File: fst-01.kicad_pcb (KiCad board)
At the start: 2 copper layers, 26.5 x 13.1 mm, 25 parts, among them J1 USB_A, K1 CONN_3, K2 CONN_2, K3 CONN_2, U1 STM32F103TB, U2 LP2985-33DBVR, U3 NUF2221W1, U4 SST25VF032B, X1 12MHz

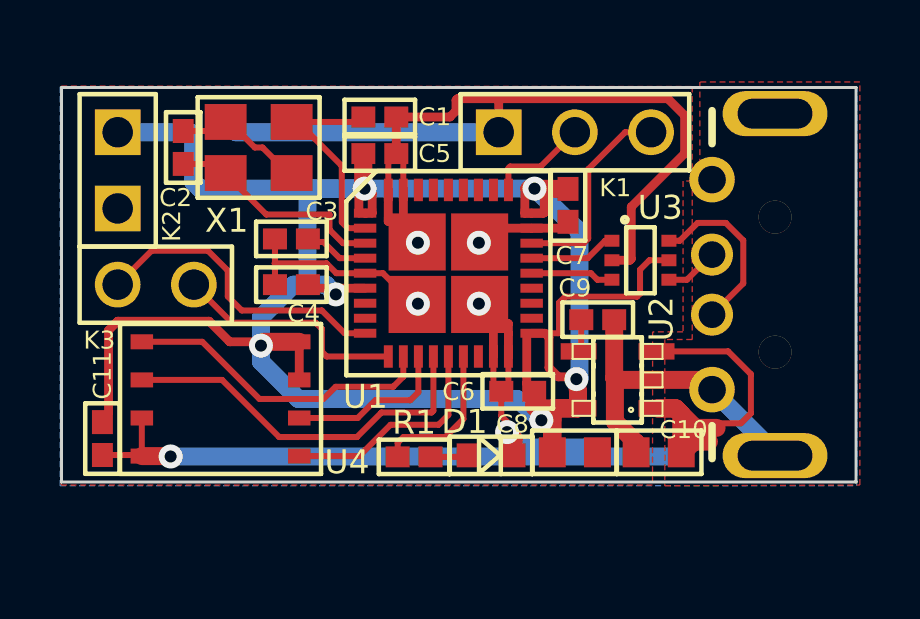
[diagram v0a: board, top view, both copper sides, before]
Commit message: fst-01sz.
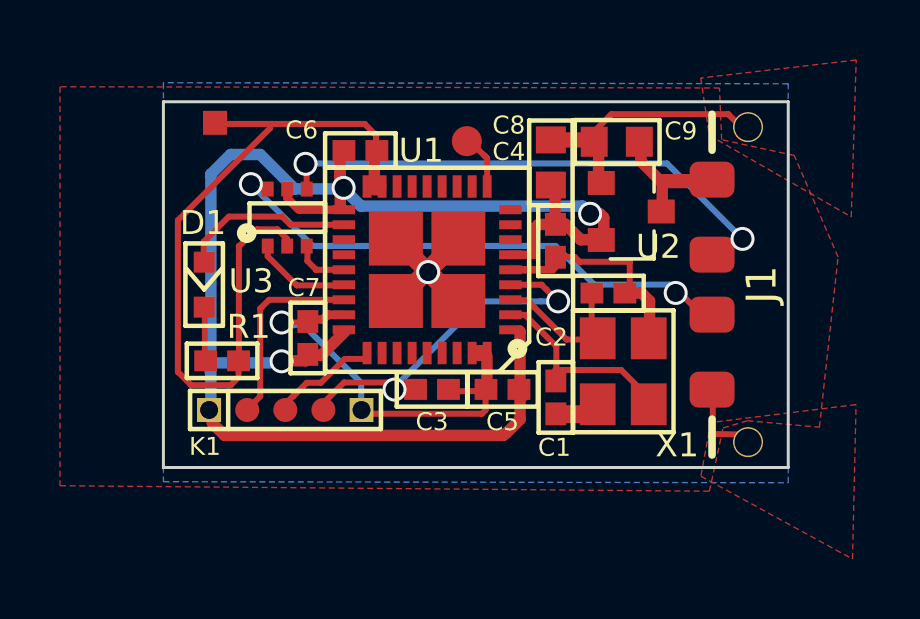
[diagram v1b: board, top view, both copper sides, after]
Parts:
- removed C10: 4.7uF, FST:c_0603
- removed C11: 0.1uF, FST:c_0402
- removed CE_mark: Symbol_CE_SilkScreen_5mm, Symbols:Symbol_CE_SilkScreen_5mm
- removed K2: CONN_2, SIL-2-0
- removed K3: CONN_2, SIL-2-2
- removed REF***: WEEE-Logo_4.2x6mm_SilkScreen, FST:WEEE-Logo_4.2x6mm_SilkScreen
- removed U4: SST25VF032B, WSON8
- added REF**: pad2, FST:pad1, F.Cu at (110.4, 93.6)
- added REF**: pad1, FST:pad1, F.Cu at (118.8, 94.2)
- C9: value 0.01uF -> 4.7uF; footprint FST:c_0402 -> FST:c_0603
- FST-LOGO: footprint FST-LOGO -> FST:FST-LOGO
- J1: footprint FST:USB-A-PLUG -> FST:USB-A-ZT01
- K1: footprint SIL-3-2 -> FST:SIL-5
- U2: value LP2985-33DBVR -> MCP1700-3302E; footprint FST:SOT23-5 -> Package_TO_SOT_SMD:SOT-23
- U3: footprint SOT363 -> FST:SOT363
- moved C2 15.0 mm to (123.5, 99.3), turned to 180 degrees
- moved X1 14.3 mm to (124.0, 101.9), turned to 90 degrees
- moved K1 13.4 mm to (112.8, 103.2)
- moved U3 11.9 mm to (112.8, 96.8), turned to 0 degrees
- moved D1 11.1 mm to (110.1, 99.0), turned to 270 degrees
- moved C1 11.0 mm to (121.8, 102.8), turned to 90 degrees
- moved C7 9.74 mm to (113.5, 100.8), turned to 90 degrees
- moved C8 9.69 mm to (121.6, 94.9), turned to 270 degrees
- moved C6 9.59 mm to (115.3, 94.5), turned to 0 degrees
- moved C4 8.92 mm to (121.8, 97.5), turned to 270 degrees
- moved C5 8.86 mm to (120.0, 102.5), turned to 180 degrees
- moved FST-LOGO 7.71 mm to (117.6, 98.6)
- moved R1 7.16 mm to (110.7, 101.5), turned to 180 degrees
- moved C3 6.86 mm to (117.7, 102.5), turned to 180 degrees
- moved C9 5.96 mm to (123.8, 94.2), turned to 0 degrees
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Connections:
- C9 pad 1: Net-(C9-Pad1) -> /VBUS
- D1 pad 1: GND -> Net-(D1-Pad1)
- D1 pad 2: Net-(D1-Pad2) -> /LED
- K1 pad 1: GND -> +3V3
- K1 pad 2: /SWCLK -> /SWDIO
- K1 pad 3: /SWDIO -> /SWCLK
- R1 pad 1: Net-(D1-Pad2) -> Net-(D1-Pad1)
- R1 pad 2: /LED -> GND
- U1 pad 10: /PA3 -> Net-(U1-Pad10)
- U1 pad 11: /NSS -> Net-(U1-Pad11)
- U1 pad 12: /CLK -> Net-(U1-Pad12)
- U1 pad 13: /MISO -> Net-(U1-Pad13)
- U1 pad 14: /MOSI -> Net-(U1-Pad14)
- U1 pad 15: /LED -> Net-(U1-Pad15)
- U1 pad 16: (no net) -> Net-(U1-Pad16)
- U1 pad 20: (no net) -> /LED
- U1 pad 21: (no net) -> Net-(U1-Pad21)
- U1 pad 22: (no net) -> Net-(U1-Pad22)
- U1 pad 29: (no net) -> Net-(U1-Pad29)
- U1 pad 30: (no net) -> Net-(U1-Pad30)
- U1 pad 31: (no net) -> Net-(U1-Pad31)
- U1 pad 32: (no net) -> Net-(U1-Pad32)
- U1 pad 33: (no net) -> Net-(U1-Pad33)
- U1 pad 34: (no net) -> Net-(U1-Pad34)
- U1 pad 7: (no net) -> Net-(U1-Pad7)
- U1 pad 8: (no net) -> Net-(U1-Pad8)
- U1 pad 9: /PA2 -> Net-(U1-Pad9)
- U2 pad 1: /VBUS -> GND
- U2 pad 2: GND -> +3V3
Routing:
- net +3V3: track 87.6 -> 53.1 mm, vias 6 -> 3
- net GND: track 94.2 -> 68.8 mm, vias 6 -> 2
- net /D-_PLUG: track 1.78 -> 18.2 mm, vias 0 -> 2
- net /MISO: track 12.7 -> 0.00 mm
- net /D+_PLUG: track 5.87 -> 17.8 mm, vias 0 -> 2
- net /NSS: track 10.5 -> 0.00 mm
- net /PA2: track 10.4 -> 0.00 mm
- net /NRST: track 2.17 -> 12.4 mm, vias 0 -> 2
- net /PA3: track 7.92 -> 0.00 mm
- net /MOSI: track 7.49 -> 0.00 mm
- net /VBUS: track 13.7 -> 6.37 mm
- net /CLK: track 5.52 -> 0.00 mm
- net Net-(U1-Pad10): track 0.00 -> 1.95 mm
- net /OSC_OUT: track 7.98 -> 6.38 mm
- net Net-(D1-Pad1): track 0.00 -> 1.41 mm
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- removed copper zone on F.Cu, net /VBUS
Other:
- board size 26.5 x 13.1 mm -> 20.8 x 12.2 mm
- rule pad_to_mask_clearance: 0.1524 -> 0.0762
- board text added: "FST-01SZ"
- board text removed: "FST-01G"

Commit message: More change.
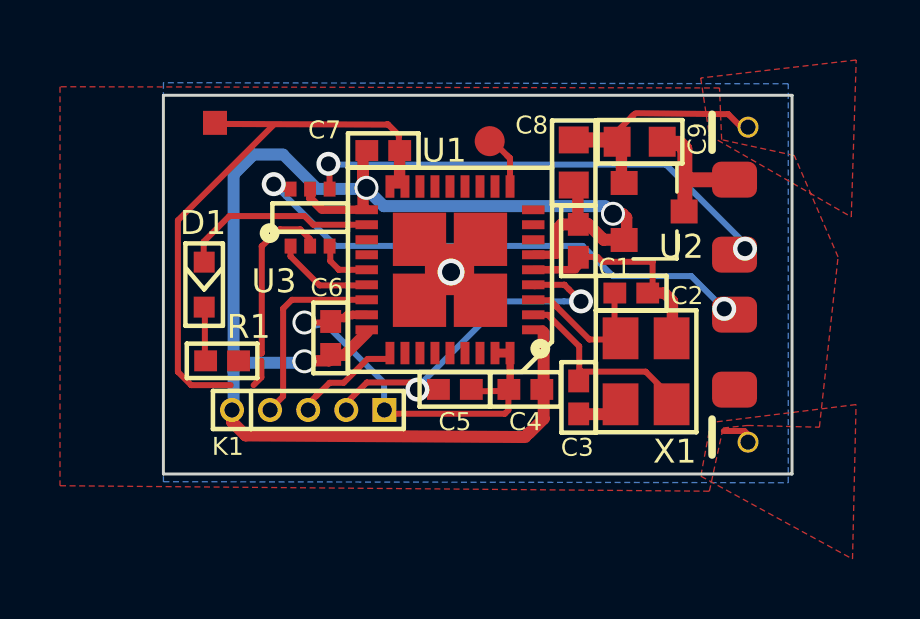
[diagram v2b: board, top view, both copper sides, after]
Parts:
- removed the C4 at (121.8, 97.5)
- added C1: 0.1uF, FST:c_0402, F.Cu at (122.5, 97.5)
- moved C7 6.74 mm to (116.0, 94.5), turned to 0 degrees
- moved C6 6.33 mm to (114.3, 100.8), turned to 90 degrees
- moved C2 0.76 mm to (124.3, 99.3)
- moved C3 0.76 mm to (122.6, 102.8)
- moved C4 0.76 mm to (120.8, 102.5)
- moved C5 0.76 mm to (118.4, 102.5)
- moved C8 0.76 mm to (122.4, 94.9)
- moved C9 0.76 mm to (124.6, 94.2)
- moved K1 0.76 mm to (113.5, 103.2)
- moved REF** 0.76 mm to (119.6, 94.2)
- moved U1 0.76 mm to (118.3, 98.5)
- moved U2 0.76 mm to (125.1, 96.6)
- moved U3 0.76 mm to (113.6, 96.8)
- moved X1 0.76 mm to (124.8, 101.9)
- moved FST-LOGO 0.74 mm to (118.3, 98.7)
- renumbered C1 to C3, C5 to C4, C3 to C5
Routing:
- net GND: track 68.8 -> 77.4 mm
- net /VBUS: track 6.37 -> 4.36 mm
- net /D-_PLUG: track 18.2 -> 17.1 mm
- net /LED: track 5.85 -> 6.59 mm
- net +3V3: track 53.1 -> 52.5 mm
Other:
- board size 20.8 x 12.2 mm -> 21 x 12.6 mm
- net class Default: via_dia 0.8001 -> 0.8; via_drill 0.59944 -> 0.5
- net class GND: via_dia 0.8001 -> 0.8; via_drill 0.59944 -> 0.5
- net class VBUS: via_dia 0.8001 -> 0.8; via_drill 0.59944 -> 0.5
- net class VDD: via_dia 0.8001 -> 0.8; via_drill 0.59944 -> 0.5
- rule trace_min: 0.20066 -> 0.2
- rule via_min_drill: 0.50038 -> 0.5
- rule via_min_size: 0.8001 -> 0.8
